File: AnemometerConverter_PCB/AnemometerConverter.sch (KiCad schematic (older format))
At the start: 19 parts, among them P1 ANEMOMETER, P2 OUTPUT, P3 PCB, P4 LOGO 1, P5 LOGO 2, U1 LM339

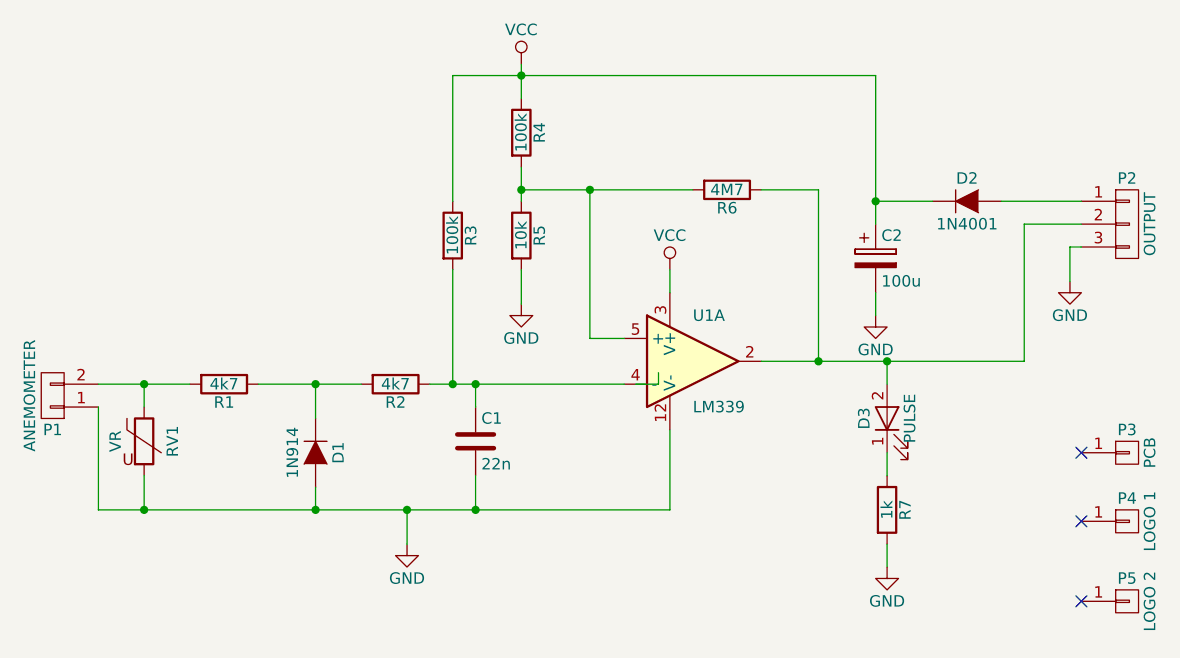
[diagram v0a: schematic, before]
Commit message: UPdated with instructions
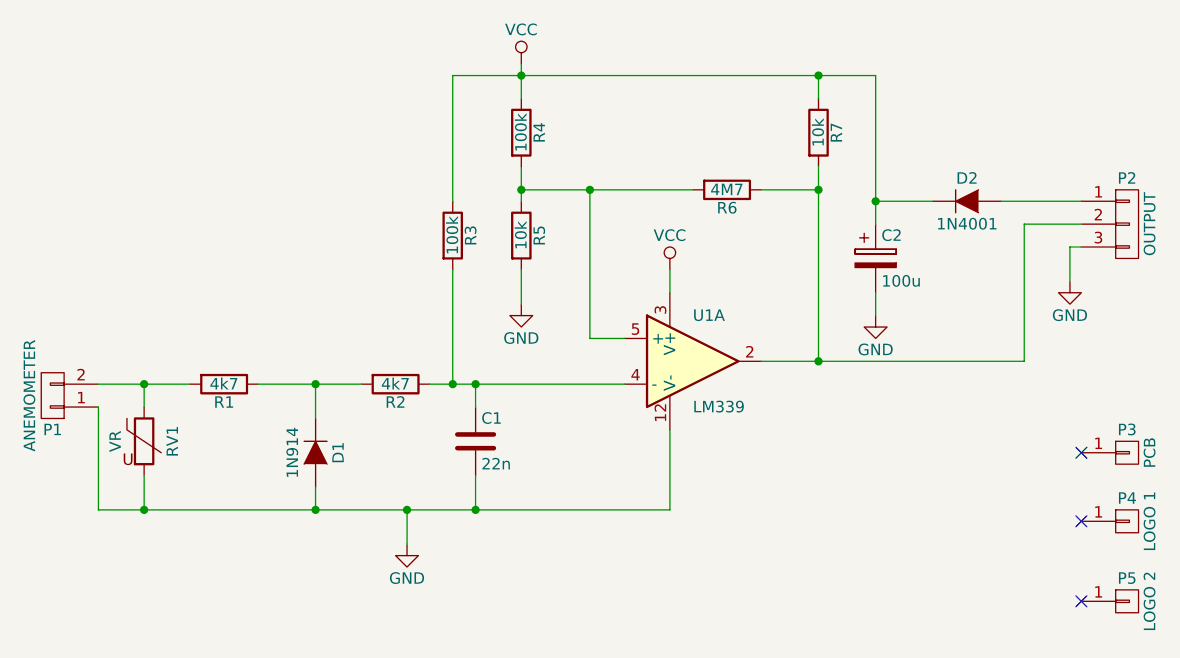
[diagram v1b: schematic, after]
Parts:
- removed D3: PULSE, REInnovationFootprint:TH_LED-5MM_larg_pad, symbol LED
- R7: value 1k -> 10k
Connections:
- wire segments 39 -> 35
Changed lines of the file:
@@
 LIBS:contrib
 LIBS:valves
+LIBS:AnemometerConverter-cache
 EELAYER 25 0
 EELAYER END
@@
 	6150 1900 6400 1900
 Wire Wire Line
-	6400 1900 6400 2650
+	6400 1800 6400 2650
 Wire Wire Line
 	6150 2650 7300 2650
@@
 Wire Wire Line
 	7500 2150 7500 2300
-$Comp
-L LED D3
-U 1 1 5ABEA7B5
-P 6700 2900
-F 0 "D3" H 6700 3000 50  0000 C CNN
-F 1 "PULSE" H 6700 2800 50  0000 C CNN
-F 2 "REInnovationFootprint:TH_LED-5MM_larg_pad" H 6700 2900 50  0001 C CNN
-F 3 "" H 6700 2900 50  0000 C CNN
-	1    6700 2900
-	0    -1   -1   0
-$EndComp
-$Comp
-L R R7
-U 1 1 5ABEA82A
-P 6700 3300
-F 0 "R7" V 6780 3300 50  0000 C CNN
-F 1 "1k" V 6700 3300 50  0000 C CNN
-F 2 "REInnovationFootprint:TH_Resistor_1" V 6630 3300 50  0001 C CNN
-F 3 "" H 6700 3300 50  0000 C CNN
-	1    6700 3300
-	1    0    0    -1
-$EndComp
-$Comp
-L GND #PWR07
-U 1 1 5ABEA8AC
-P 6700 3550
-F 0 "#PWR07" H 6700 3300 50  0001 C CNN
-F 1 "GND" H 6700 3400 50  0000 C CNN
-F 2 "" H 6700 3550 50  0000 C CNN
-F 3 "" H 6700 3550 50  0000 C CNN
-	1    6700 3550
-	1    0    0    -1
-$EndComp
-Wire Wire Line
-	6700 2750 6700 2650
-Connection ~ 6700 2650
-Wire Wire Line
-	6700 3050 6700 3150
-Wire Wire Line
-	6700 3450 6700 3550
 $Comp
 L CONN_01X01 P3
@@
 Wire Wire Line
 	6900 1950 6650 1950
-Wire Wire Line
-	5600 2750 5700 2750
-Wire Wire Line
-	5700 2750 5700 2700
+$Comp
+L R R7
+U 1 1 5AE4A1C3
+P 6400 1650
+F 0 "R7" V 6480 1650 50  0000 C CNN
+F 1 "10k" V 6400 1650 50  0000 C CNN
+F 2 "REInnovationFootprint:TH_Resistor_1" V 6330 1650 50  0001 C CNN
+F 3 "" H 6400 1650 50  0000 C CNN
+	1    6400 1650
+	1    0    0    -1
+$EndComp
+Connection ~ 6400 1900
+Wire Wire Line
+	6400 1500 6400 1400
+Connection ~ 6400 1400
 $EndSCHEMATC
